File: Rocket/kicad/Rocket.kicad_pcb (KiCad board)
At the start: 2 copper layers, 135.2 x 112.1 mm, 35 parts, among them Q1 Q_NPN_EBC, Q2 Q_NPN_EBC, U1 NE555P, U2 BAT_HLD_SMD

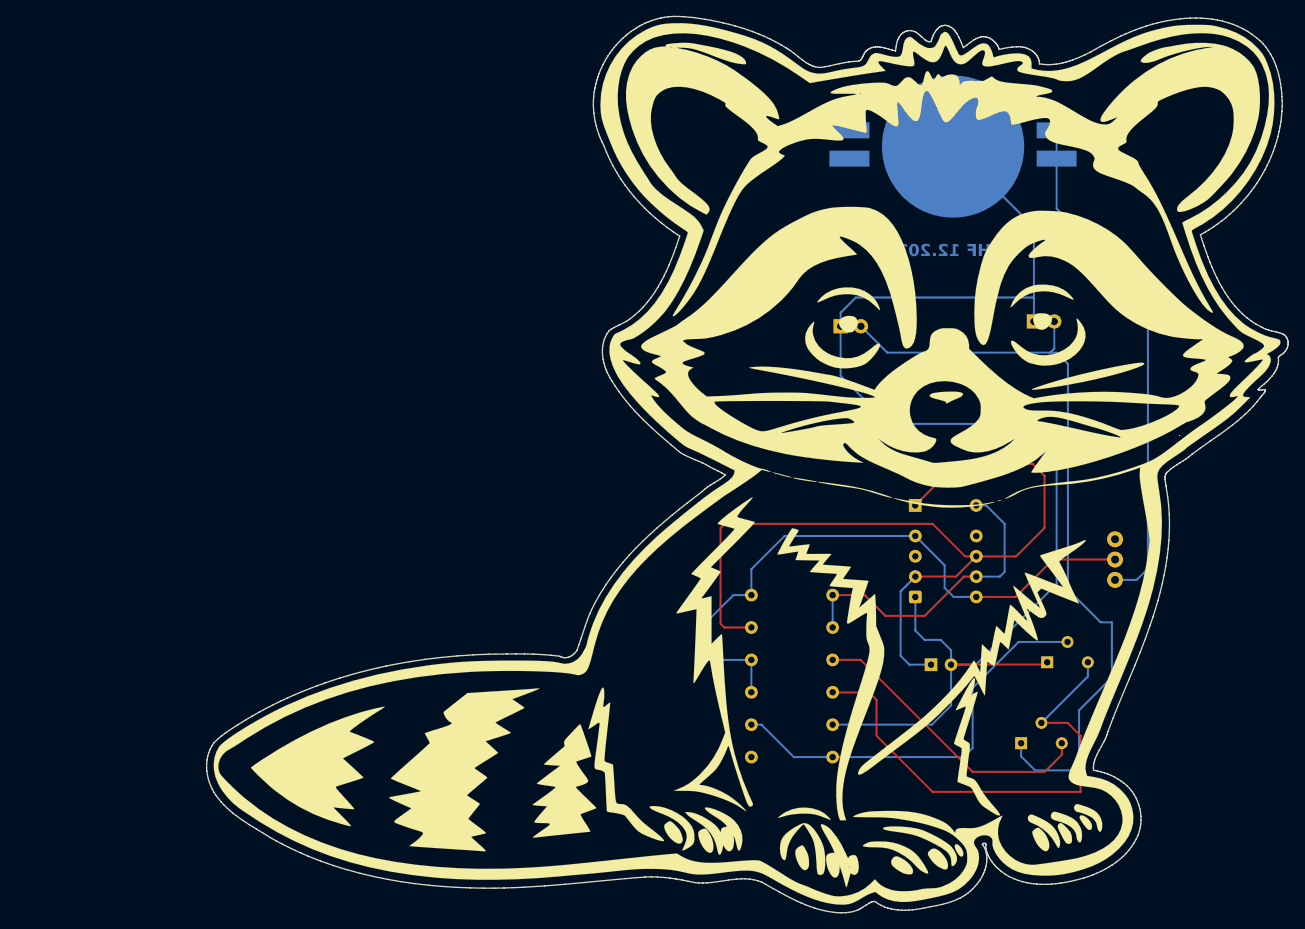
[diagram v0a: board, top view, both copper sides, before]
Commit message: V03012026
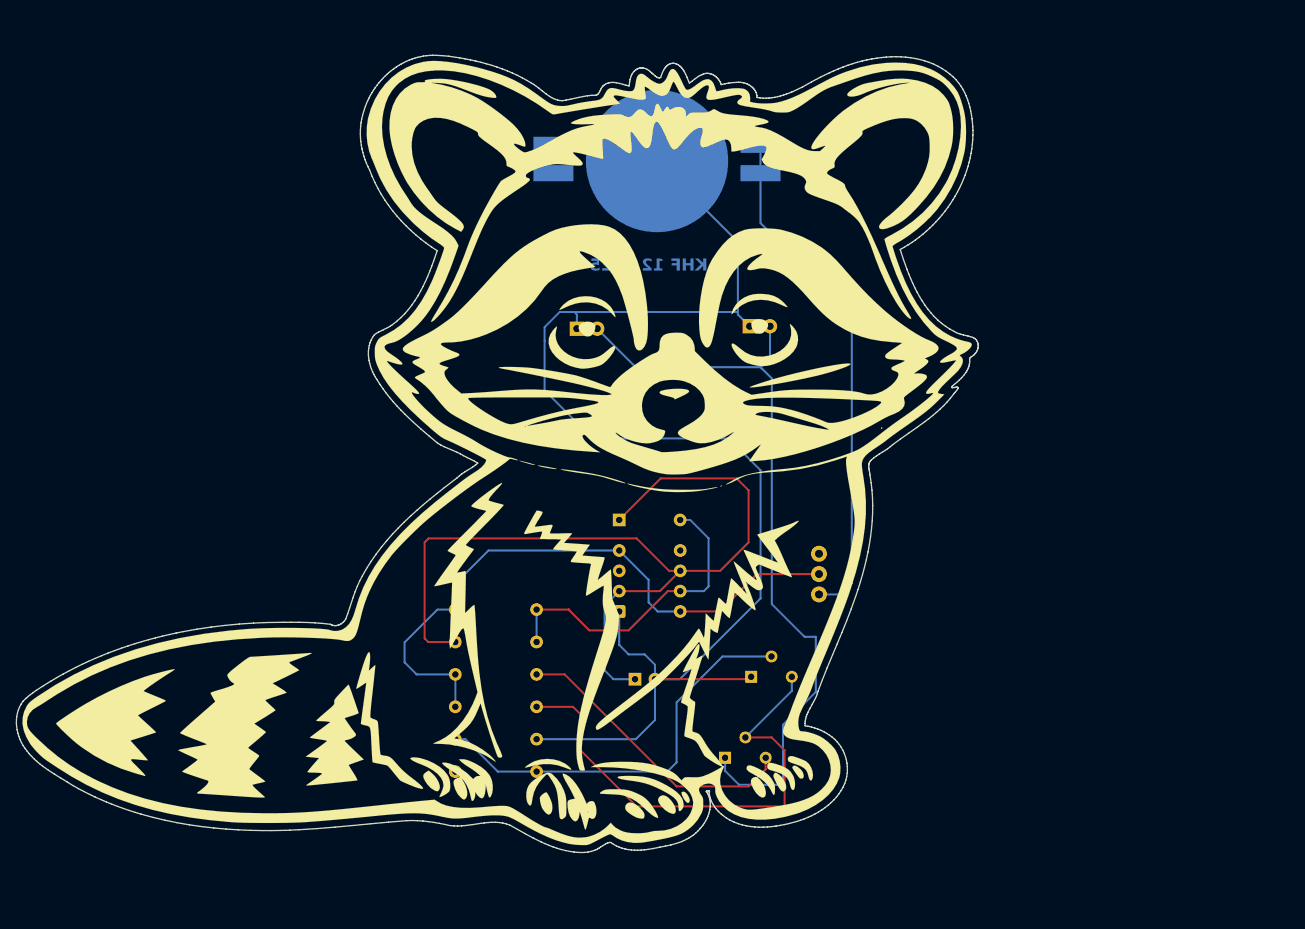
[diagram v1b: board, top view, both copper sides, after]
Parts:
- removed the G*** at (131.6, 96.3) (x7)
- removed the G*** at (136.6, 104.1) (x6)
- removed the G*** at (136.4, 104.1) (x6)
- added G*** (x6): LOGO, LOGO, F.Cu at (99.6, 105.9)
- added G*** (x6): LOGO, LOGO, F.Cu at (94.6, 98.1)
- added G*** (x6): LOGO, LOGO, F.Cu at (99.4, 105.9)
- added G*** (x7): LOGO, LOGO, F.Cu at (108.0, 101.2)
- moved Q2 37.1 mm to (123.9, 133.0)
- moved U2 37.1 mm to (115.3, 58.4)
- moved Q1 37.1 mm to (127.1, 122.9)
- moved R3 37.1 mm to (90.1, 134.8)
- moved R4 37.1 mm to (90.1, 130.7)
- moved R5 37.1 mm to (90.1, 126.7)
- moved R6 37.1 mm to (90.1, 122.6)
- moved R7 37.1 mm to (90.1, 118.6)
- moved R8 37.1 mm to (90.1, 114.5)
- moved S1 37.1 mm to (135.6, 112.6)
- moved U1 37.1 mm to (110.6, 114.7)
- moved C1 37.1 mm to (112.6, 123.2)
- moved D3 37.1 mm to (110.6, 103.3)
- moved G*** 37.0 mm to (121.9, 105.5)
- moved D1 35.5 mm to (126.9, 79.1)
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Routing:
- net Net-(D1-A): track 97.1 -> 95.2 mm
- net Net-(D1-K): track 168.0 -> 169.6 mm
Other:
- board size 135.2 x 112.1 mm -> 120.2 x 99.7 mm
